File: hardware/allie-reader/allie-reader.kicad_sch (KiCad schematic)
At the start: 17 parts, among them J1 8P8C Socket, J2 Reader, U1 MAX488E, U2 LD1117S50TR, U3 CH32V003JxMx

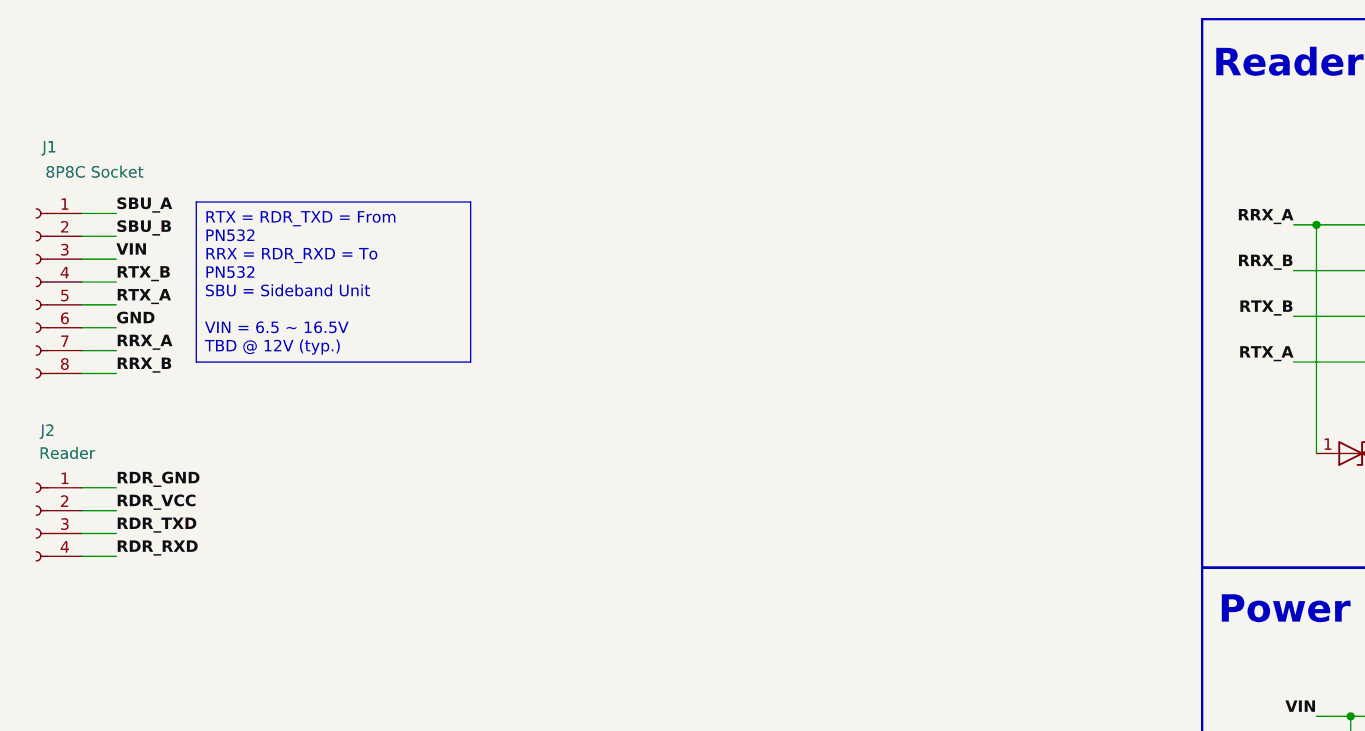
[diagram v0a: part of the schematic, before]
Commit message: hw/reader: drafts
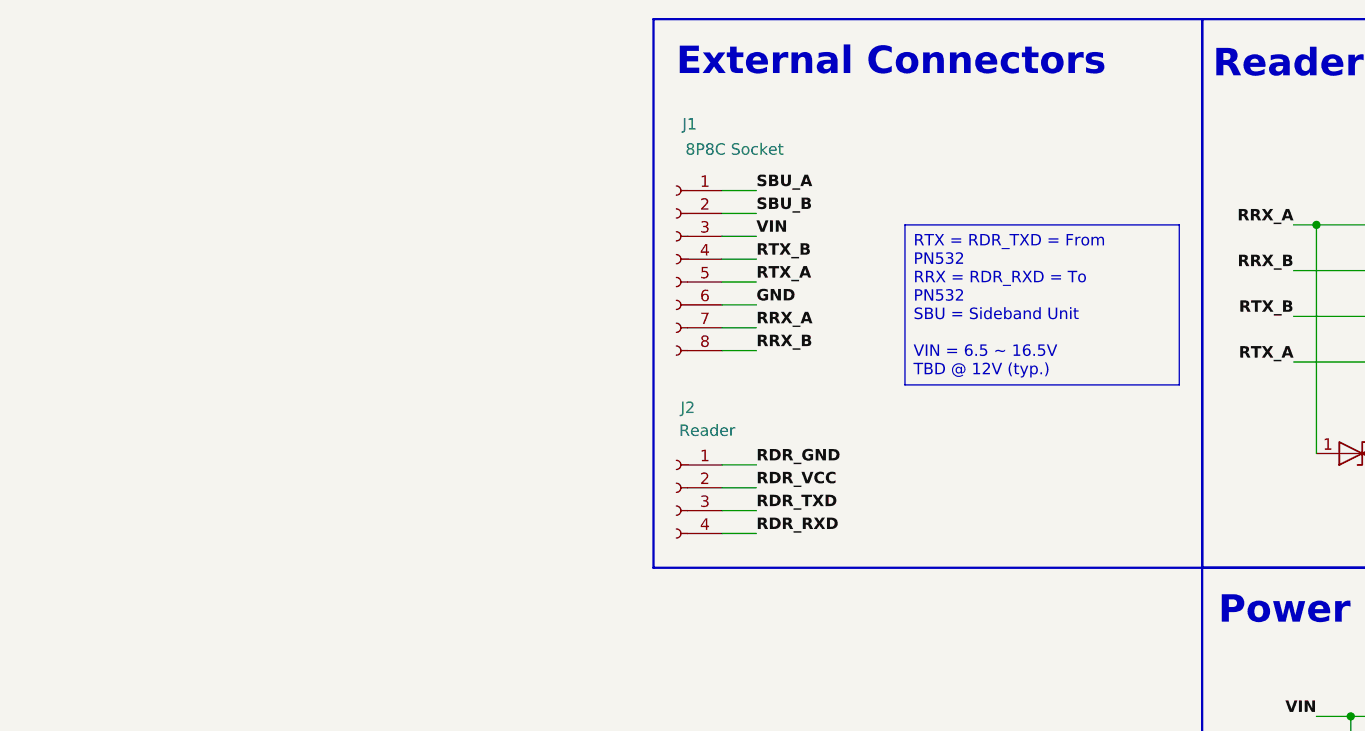
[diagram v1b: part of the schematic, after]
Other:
- note added: "External Connectors"
- moved on the sheet: J1, J2
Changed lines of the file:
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@@
+	)
+	(rectangle
+		(start 96.52 20.32)
+		(end 157.48 81.28)
+		(stroke
+			(width 0.254)
+			(type solid)
+		)
+		(fill
+			(type none)
+		)
 	)
 	(rectangle
@@
 		)
 	)
+	(text "External Connectors"
+		(exclude_from_sim no)
+		(at 122.936 25.146 0)
+		(effects
+			(font
+				(size 3.048 3.048)
+				(thickness 0.762)
+				(bold yes)
+			)
+		)
+	)
 	(text "Power"
 		(exclude_from_sim no)
@@
 	(text_box "RTX = RDR_TXD = From PN532\nRRX = RDR_RXD = To PN532\nSBU = Sideband Unit\n\nVIN = 6.5 ~ 16.5V\nTBD @ 12V (typ.)"
 		(exclude_from_sim no)
-		(at 45.72 40.64 0)
+		(at 124.46 43.18 0)
 		(size 30.48 17.78)
 		(margins 0.9525 0.9525 0.9525 0.9525)
@@
 	(wire
 		(pts
-			(xy 33.02 41.91) (xy 36.83 41.91)
-		)
-		(stroke
-			(width 0)
-			(type default)
-		)
-	)
-	(wire
-		(pts
-			(xy 33.02 49.53) (xy 36.83 49.53)
+			(xy 104.14 39.37) (xy 107.95 39.37)
+		)
+		(stroke
+			(width 0)
+			(type default)
+		)
+	)
+	(wire
+		(pts
+			(xy 104.14 46.99) (xy 107.95 46.99)
 		)
 		(stroke
@@
 	(wire
 		(pts
-			(xy 33.02 52.07) (xy 36.83 52.07)
+			(xy 104.14 49.53) (xy 107.95 49.53)
 		)
 		(stroke
@@
 	(wire
 		(pts
-			(xy 33.02 57.15) (xy 36.83 57.15)
+			(xy 104.14 54.61) (xy 107.95 54.61)
 		)
 		(stroke
@@
 	(wire
 		(pts
-			(xy 33.02 44.45) (xy 36.83 44.45)
+			(xy 104.14 41.91) (xy 107.95 41.91)
 		)
 		(stroke
@@
 	(wire
 		(pts
-			(xy 33.02 54.61) (xy 36.83 54.61)
+			(xy 104.14 52.07) (xy 107.95 52.07)
 		)
 		(stroke
@@
 	(wire
 		(pts
-			(xy 36.83 72.39) (xy 33.02 72.39)
+			(xy 107.95 69.85) (xy 104.14 69.85)
 		)
 		(stroke
@@
 	(wire
 		(pts
-			(xy 33.02 59.69) (xy 36.83 59.69)
+			(xy 104.14 57.15) (xy 107.95 57.15)
 		)
 		(stroke
@@
 	(wire
 		(pts
-			(xy 36.83 80.01) (xy 33.02 80.01)
+			(xy 107.95 77.47) (xy 104.14 77.47)
 		)
 		(stroke
@@
 	(wire
 		(pts
-			(xy 33.02 46.99) (xy 36.83 46.99)
+			(xy 104.14 44.45) (xy 107.95 44.45)
 		)
 		(stroke
@@
 	(wire
 		(pts
-			(xy 36.83 74.93) (xy 33.02 74.93)
+			(xy 107.95 72.39) (xy 104.14 72.39)
 		)
 		(stroke
@@
 	(wire
 		(pts
-			(xy 36.83 77.47) (xy 33.02 77.47)
+			(xy 107.95 74.93) (xy 104.14 74.93)
 		)
 		(stroke
@@
 	)
 	(label "RRX_B"
-		(at 36.83 59.69 0)
+		(at 107.95 57.15 0)
 		(effects
 			(font
@@
 	)
 	(label "GND"
-		(at 36.83 54.61 0)
+		(at 107.95 52.07 0)
 		(effects
 			(font
@@
 	)
 	(label "RDR_VCC"
-		(at 36.83 74.93 0)
+		(at 107.95 72.39 0)
 		(effects
 			(font
@@
 	)
 	(label "RDR_TXD"
-		(at 36.83 77.47 0)
+		(at 107.95 74.93 0)
 		(effects
 			(font
@@
 	)
 	(label "RTX_A"
-		(at 36.83 52.07 0)
+		(at 107.95 49.53 0)
 		(effects
 			(font
@@
 	)
 	(label "RDR_GND"
-		(at 36.83 72.39 0)
+		(at 107.95 69.85 0)
 		(effects
 			(font
@@
 	)
 	(label "RTX_B"
-		(at 36.83 49.53 0)
+		(at 107.95 46.99 0)
 		(effects
 			(font
@@
 	)
 	(label "SBU_B"
-		(at 36.83 44.45 0)
+		(at 107.95 41.91 0)
 		(effects
 			(font
@@
 	)
 	(label "RRX_A"
-		(at 36.83 57.15 0)
+		(at 107.95 54.61 0)
 		(effects
 			(font
@@
 	)
 	(label "SBU_A"
-		(at 36.83 41.91 0)
+		(at 107.95 39.37 0)
 		(effects
 			(font
@@
 	)
 	(label "VIN"
-		(at 36.83 46.99 0)
+		(at 107.95 44.45 0)
 		(effects
 			(font
@@
 	)
 	(label "RDR_RXD"
-		(at 36.83 80.01 0)
+		(at 107.95 77.47 0)
 		(effects
 			(font
@@
 	(symbol
 		(lib_id "Connector:Conn_01x04_Socket")
-		(at 27.94 74.93 0)
+		(at 99.06 72.39 0)
 		(mirror y)
 		(unit 1)
@@
 		(dnp no)
 		(property "Reference" "J2"
-			(at 29.21 66.04 0)
+			(at 100.33 63.5 0)
 			(effects
 				(font
@@
 		)
 		(property "Value" "Reader"
-			(at 31.369 68.58 0)
+			(at 102.489 66.04 0)
 			(effects
 				(font
@@
 		)
 		(property "Footprint" "Connector_PinSocket_2.54mm:PinSocket_1x04_P2.54mm_Vertical"
-			(at 27.94 74.93 0)
+			(at 99.06 72.39 0)
 			(effects
 				(font
@@
 		)
 		(property "Datasheet" "~"
-			(at 27.94 74.93 0)
+			(at 99.06 72.39 0)
 			(effects
 				(font
@@
 		)
 		(property "Description" "Generic connector, single row, 01x04, script generated"
-			(at 27.94 74.93 0)
+			(at 99.06 72.39 0)
 			(effects
 				(font
@@
 	(symbol
 		(lib_id "Connector:Conn_01x08_Socket")
-		(at 27.94 49.53 0)
+		(at 99.06 46.99 0)
 		(mirror y)
 		(unit 1)
@@
 		(dnp no)
 		(property "Reference" "J1"
-			(at 30.226 34.544 0)
+			(at 101.346 32.004 0)
 			(effects
 				(font
@@
 		)
 		(property "Value" "8P8C Socket"
-			(at 39.878 37.338 0)
+			(at 110.998 34.798 0)
 			(effects
 				(font
@@
 		)
 		(property "Footprint" ""
-			(at 27.94 49.53 0)
+			(at 99.06 46.99 0)
 			(effects
 				(font
@@
 		)
 		(property "Datasheet" "~"
-			(at 27.94 49.53 0)
+			(at 99.06 46.99 0)
 			(effects
 				(font
@@
 		)
 		(property "Description" "Generic connector, single row, 01x08, script generated"
-			(at 27.94 49.53 0)
-			(effects
-				(font
+			(at 99.06 46.99 0)
+			(effects
+				(font
